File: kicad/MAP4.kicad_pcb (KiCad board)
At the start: 2 copper layers, 9 parts, among them P2 Pin

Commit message: work in progress
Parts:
- moved P2 239.3 mm to (-0.10, -24.1)
- moved D1 239.0 mm to (0.00, -17.0)
- moved R1 238.9 mm to (0.00, -12.2)
- moved D3 238.3 mm to (-17.2, 10.0), turned to 30 degrees
- moved R2 237.9 mm to (12.5, 7.50), turned to 60 degrees
- moved G*** 237.9 mm to (-0.10, -2.40)
- moved R3 237.0 mm to (-12.5, 7.50), turned to 120 degrees
- moved D2 236.9 mm to (17.2, 10.0), turned to 150 degrees
- moved BT1 236.5 mm to (0.00, 1.00)
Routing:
- net /3V: track 0.00 -> 81.1 mm
- net /GND: track 0.00 -> 64.0 mm
- net /LED_grn: track 0.00 -> 9.40 mm
- net /LED_blu: track 0.00 -> 9.40 mm
- net /LED_red: track 0.00 -> 6.99 mm
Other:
- board outline added: 49.8 x 48.9 mm

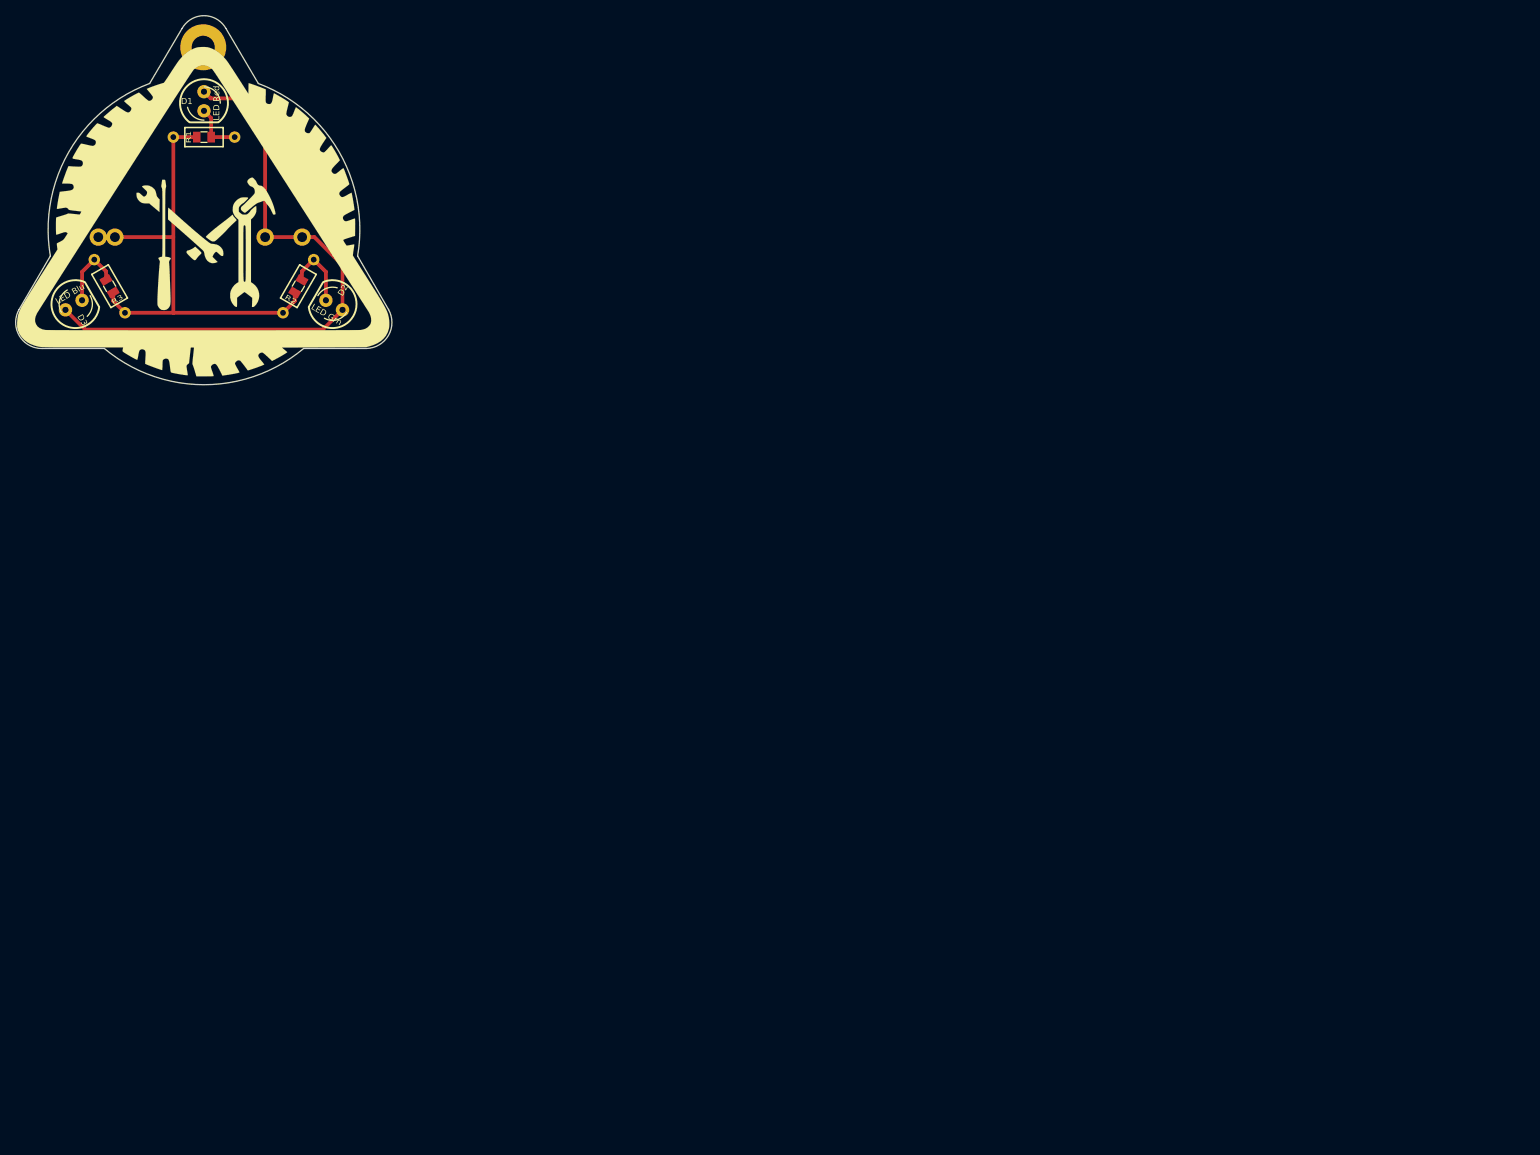
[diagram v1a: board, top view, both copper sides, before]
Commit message: MAP4 complete. Boards ordered out
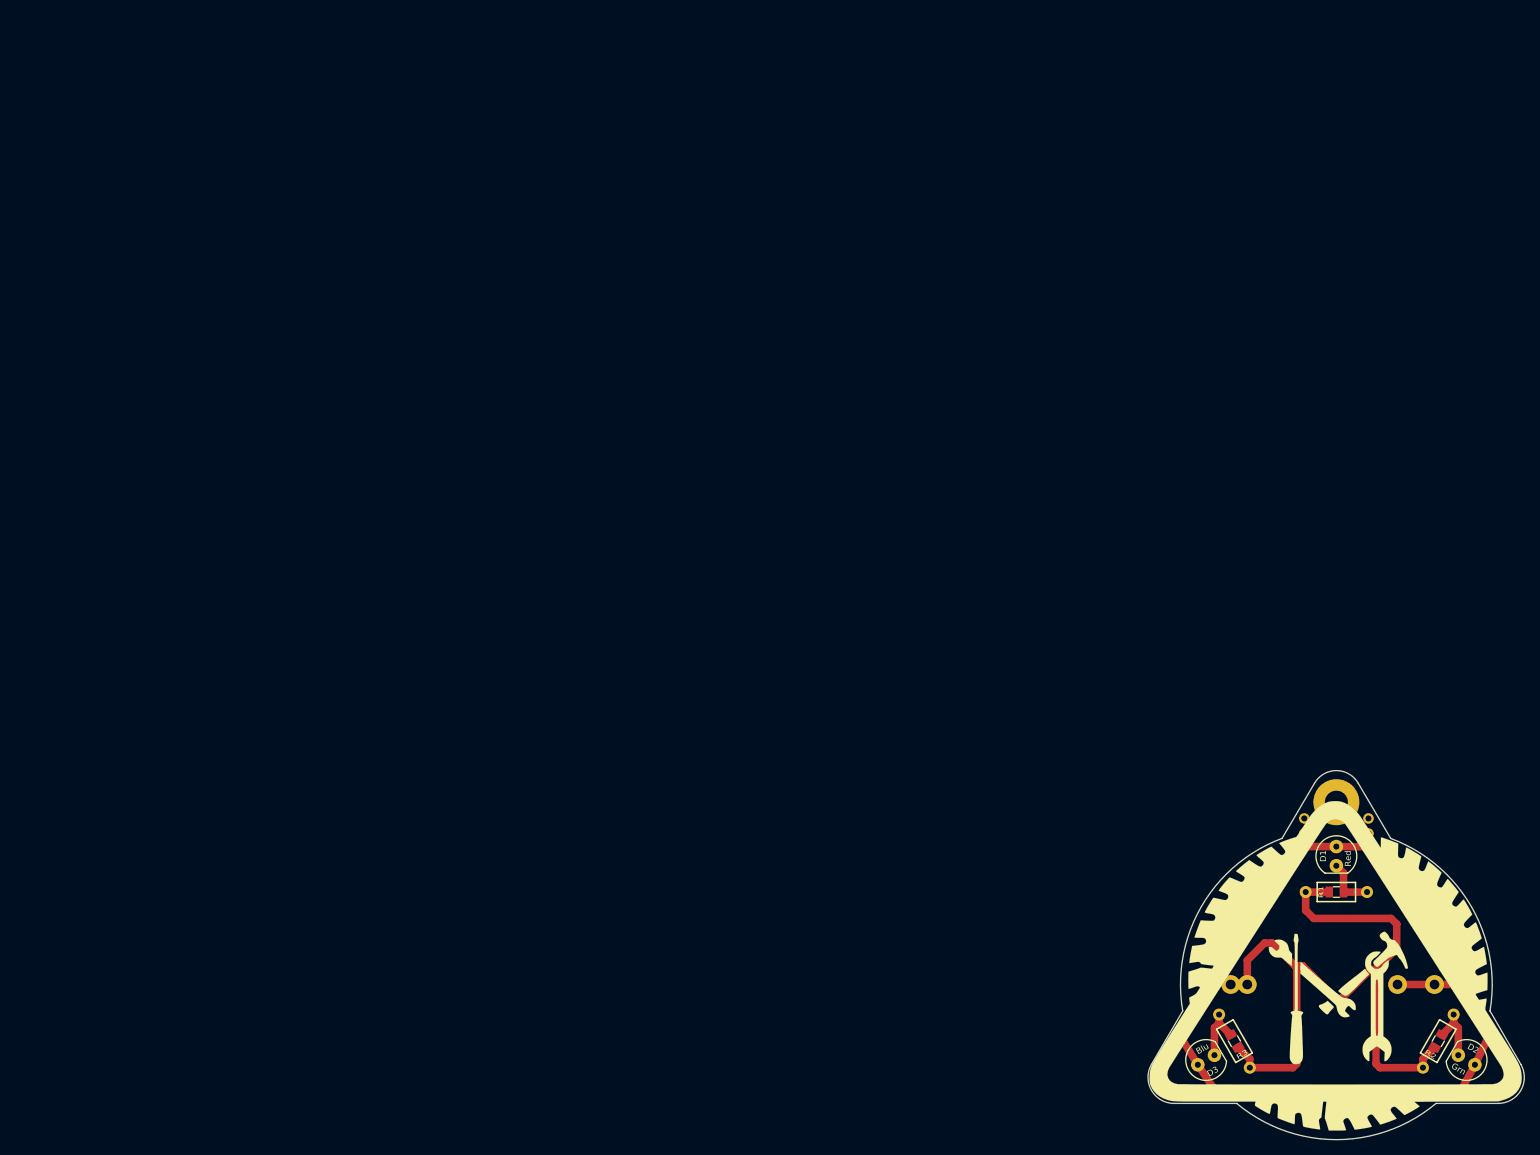
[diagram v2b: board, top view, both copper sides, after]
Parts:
- removed G***: LOGO, map4_fp:MA_LOGO4
- added LOGO1: OPEN_HARDWARE_1, map4_fp:Logo_silk_OSHW_6x6mm, B.Cu at (135.0, 112.2)
- added P1: Logo_MA, map4_fp:MA_LOGO4, F.Cu at (149.9, 97.5)
- added P3: Pin, map4_fp:MTG_0mm8, F.Cu at (145.8, 80.0)
- added P4: Pin, map4_fp:MTG_0mm8, F.Cu at (145.8, 78.0)
- added P5: Pin, map4_fp:MTG_0mm8, F.Cu at (154.2, 80.0)
- added P6: Pin, map4_fp:MTG_0mm8, F.Cu at (154.2, 78.0)
- D1: value LED Red -> Red
- D2: value LED Grn -> Grn
- D3: value LED Blu -> Blu
- moved R2 181.1 mm to (163.5, 107.5)
- moved P2 180.4 mm to (150.0, 75.8)
- moved D1 180.3 mm to (150.0, 83.0)
- moved D2 180.3 mm to (167.2, 110.0)
- moved D3 180.3 mm to (132.8, 110.0)
- moved R1 180.3 mm to (150.0, 87.8)
- moved BT1 179.7 mm to (150.0, 100.0)
- moved R3 179.4 mm to (136.5, 107.5)
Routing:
- net /3V: track 81.1 -> 126.4 mm
- net /GND: track 64.0 -> 98.9 mm
- net /LED_grn: track 9.40 -> 7.84 mm
- net /LED_blu: track 9.40 -> 7.84 mm
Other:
- board text added: "EASY"
- board text added: "HERE'S MY MAP4 SKILL BADGE"
- board text added: "IS"
- board text added: "MAKER'S ASYLUM"
- board text added: "SOLDERING"
- board text added: "[+]"
- board text added: "[-]"
